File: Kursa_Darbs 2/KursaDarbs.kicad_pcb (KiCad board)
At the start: 2 copper layers, 100.6 x 66.6 mm, 43 parts, among them J1 INPUT, J2 OUTPUT, J3 +40V, J4 -40V, Q1 MPSA43, Q2 MPSA43, Q3 BC546, Q4 MPSA43, Q5 BC546, Q6 MJE340, Q7 MJE350, Q8 IRFP240, Q9 IRFP9240

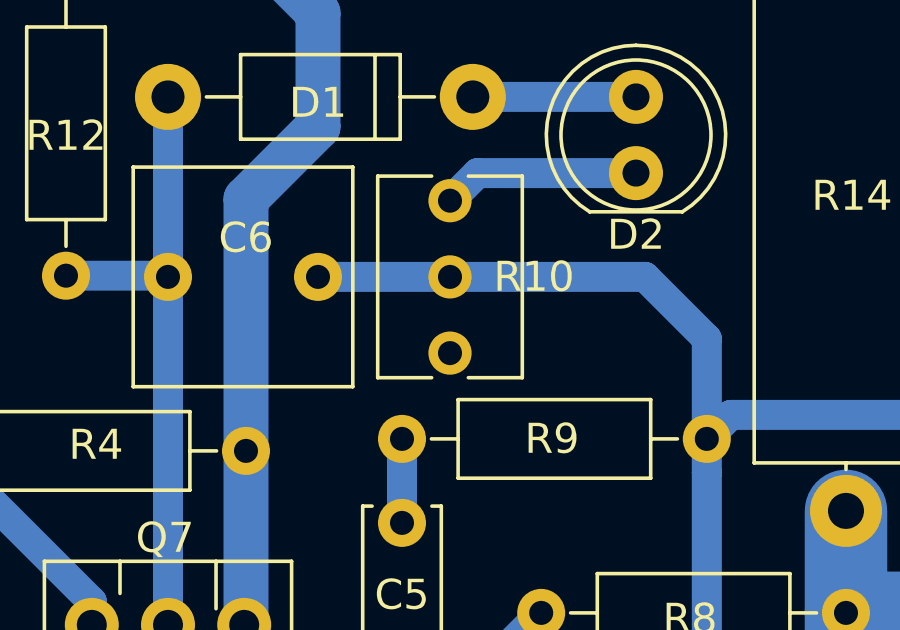
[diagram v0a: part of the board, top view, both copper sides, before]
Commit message: trimmer potentiometra labojums
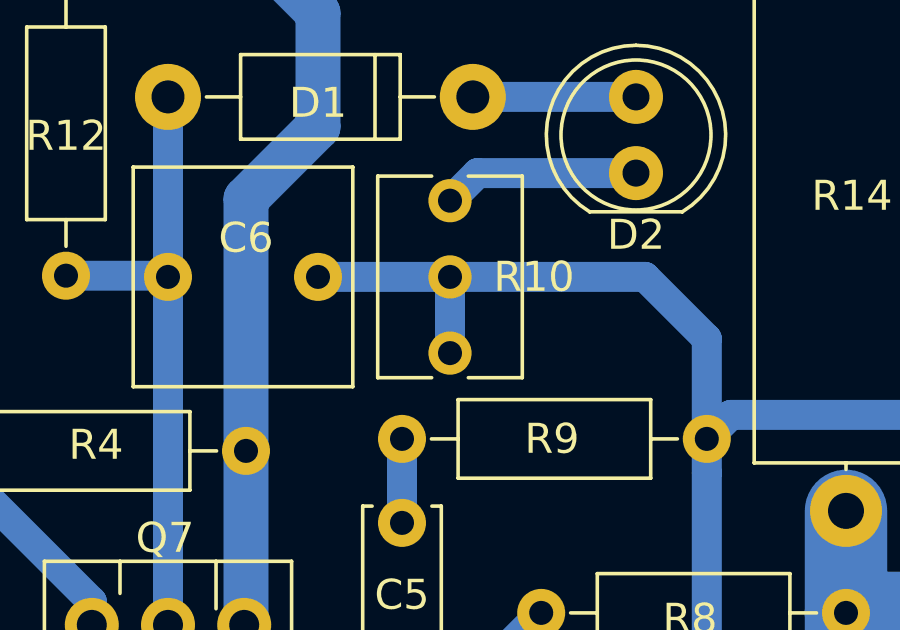
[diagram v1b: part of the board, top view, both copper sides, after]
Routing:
- net Net-(C6-Pad2): track 58.7 -> 61.2 mm
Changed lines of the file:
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@@
 (kicad_pcb (version 4) (host pcbnew 4.0.6)
   (general
-    (links 69)
-    (no_connects 0)
-    (area 72.675 59.724999 175.625 126.475001)
+    (links 70)
+    (no_connects 1)
+    (area 73.224999 59.724999 173.975001 126.475001)
     (thickness 1.6)
     (drawings 30)
-    (tracks 130)
+    (tracks 131)
     (zones 0)
     (modules 43)
@@
     (fp_line (start 2.6 6.1) (end 2.6 -1.05) (layer F.CrtYd) (width 0.05))
     (fp_line (start 2.6 -1.05) (end -2.6 -1.05) (layer F.CrtYd) (width 0.05))
-    (pad 2 thru_hole circle (at 0 5.08) (size 1.44 1.44) (drill 0.8) (layers *.Cu *.Mask))
+    (pad 2 thru_hole circle (at 0 5.08) (size 1.44 1.44) (drill 0.8) (layers *.Cu *.Mask)
+      (net 9 "Net-(C6-Pad2)"))
     (pad 2 thru_hole circle (at 0 2.54) (size 1.44 1.44) (drill 0.8) (layers *.Cu *.Mask)
       (net 9 "Net-(C6-Pad2)"))
@@
   (segment (start 113.36 78.56) (end 113.4 78.6) (width 1) (layer B.Cu) (net 8))
   (segment (start 113.4 72.6) (end 113.4 78.6) (width 1) (layer B.Cu) (net 8))
+  (segment (start 122.8 81.14) (end 122.8 78.6) (width 1) (layer B.Cu) (net 9))
   (segment (start 122.8 78.6) (end 118.4 78.6) (width 1) (layer B.Cu) (net 9))
   (segment (start 129.3 78.6) (end 122.8 78.6) (width 1) (layer B.Cu) (net 9))
